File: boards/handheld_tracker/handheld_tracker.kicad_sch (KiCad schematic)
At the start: 16 parts, among them J3 Conn_01x02_Pin, U1 SAM-M8Q, U2 RFM96W-433S2, U4 LM3670MF

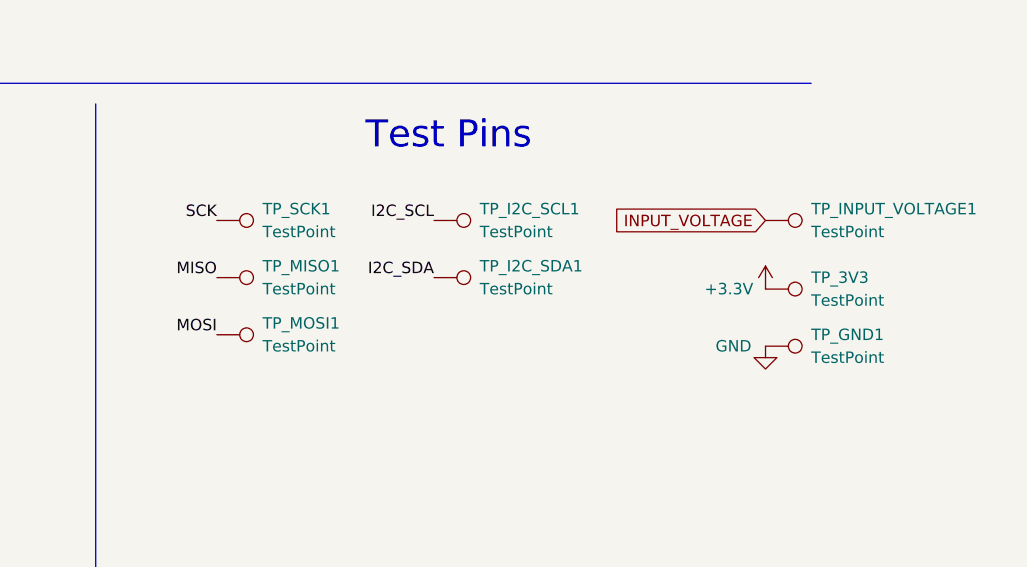
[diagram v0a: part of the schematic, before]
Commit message: finished board pre-review
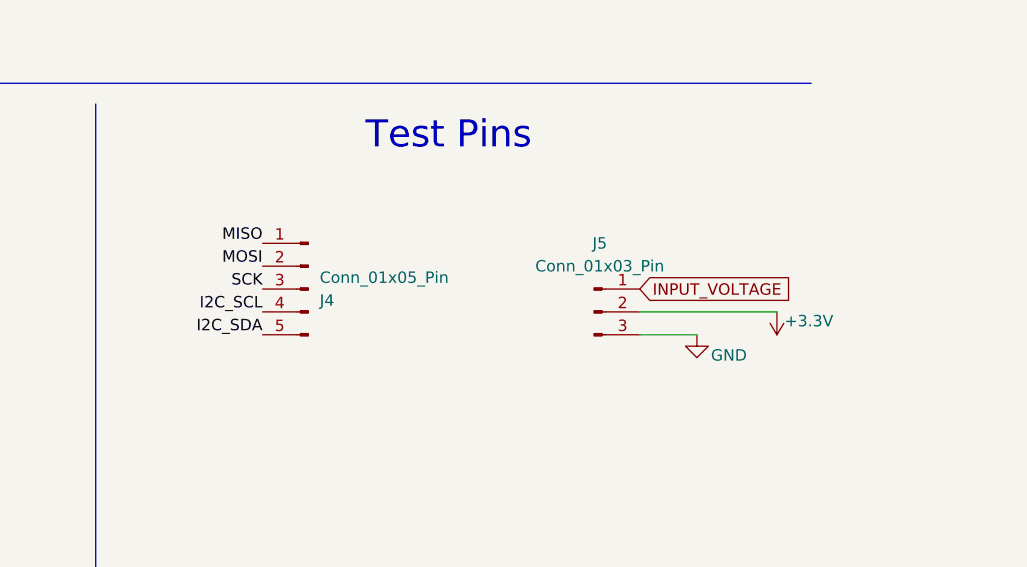
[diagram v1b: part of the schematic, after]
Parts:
- removed TP_3V3, TP_GND1, TP_I2C_SCL1, TP_I2C_SDA1, TP_INPUT_VOLTAGE1, TP_MISO1, TP_MOSI1, TP_SCK1: TestPoint, TestPoint:TestPoint_Pad_D3.0mm, symbol Connector:TestPoint
- added J4: Conn_01x05_Pin, Connector_PinHeader_2.54mm:PinHeader_1x05_P2.54mm_Vertical, symbol Connector:Conn_01x05_Pin
- added J5: Conn_01x03_Pin, Connector_PinHeader_2.54mm:PinHeader_1x03_P2.54mm_Vertical, symbol Connector:Conn_01x03_Pin
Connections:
- net +3.3V: now also J5.2 (Pin_2)
- net GND: now also J5.3 (Pin_3)
- net I2C_SCL: now also J4.4 (Pin_4)
- net I2C_SDA: now also J4.5 (Pin_5)
- net INPUT_VOLTAGE: now also J5.1 (Pin_1)
- net MISO: now also J4.1 (Pin_1)
- net MOSI: now also J4.2 (Pin_2)
- net SCK: now also J4.3 (Pin_3)
